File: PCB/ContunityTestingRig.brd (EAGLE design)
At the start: 82.8 x 65 mm, 29 parts

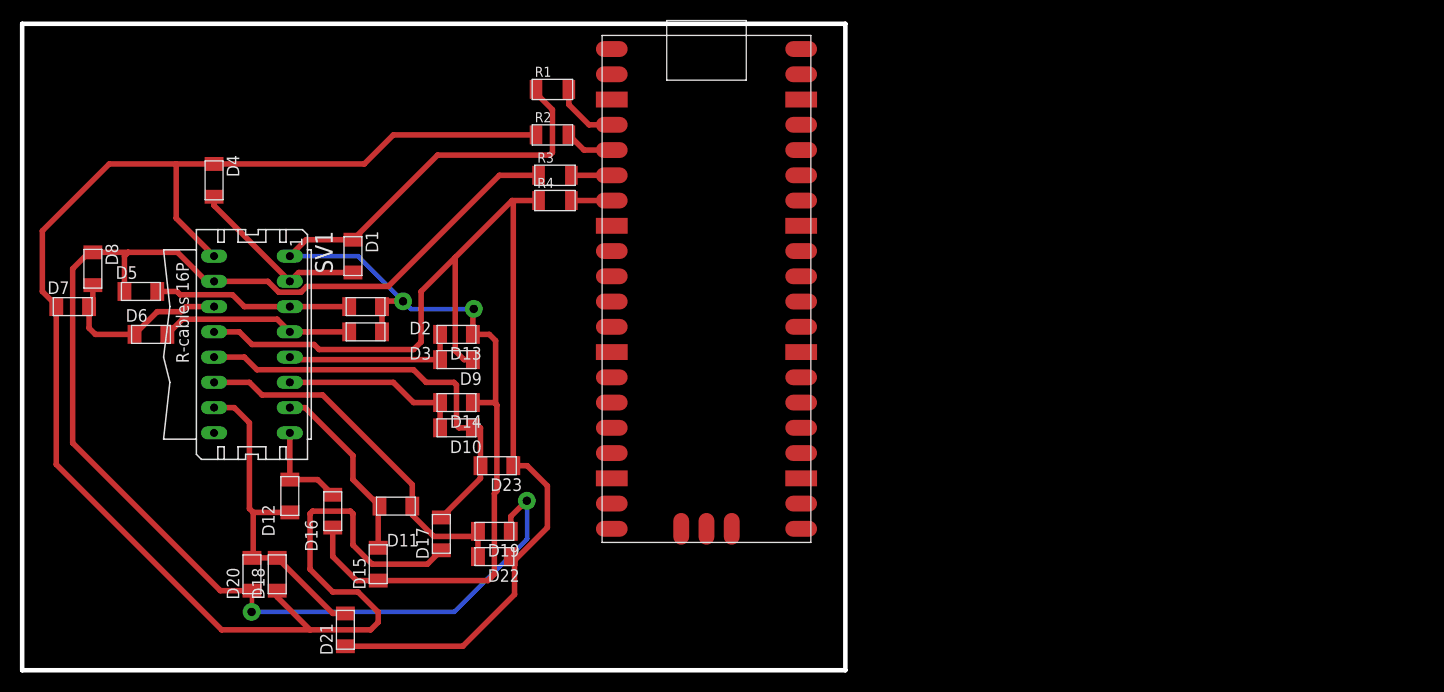
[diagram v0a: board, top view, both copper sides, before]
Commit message: Updates
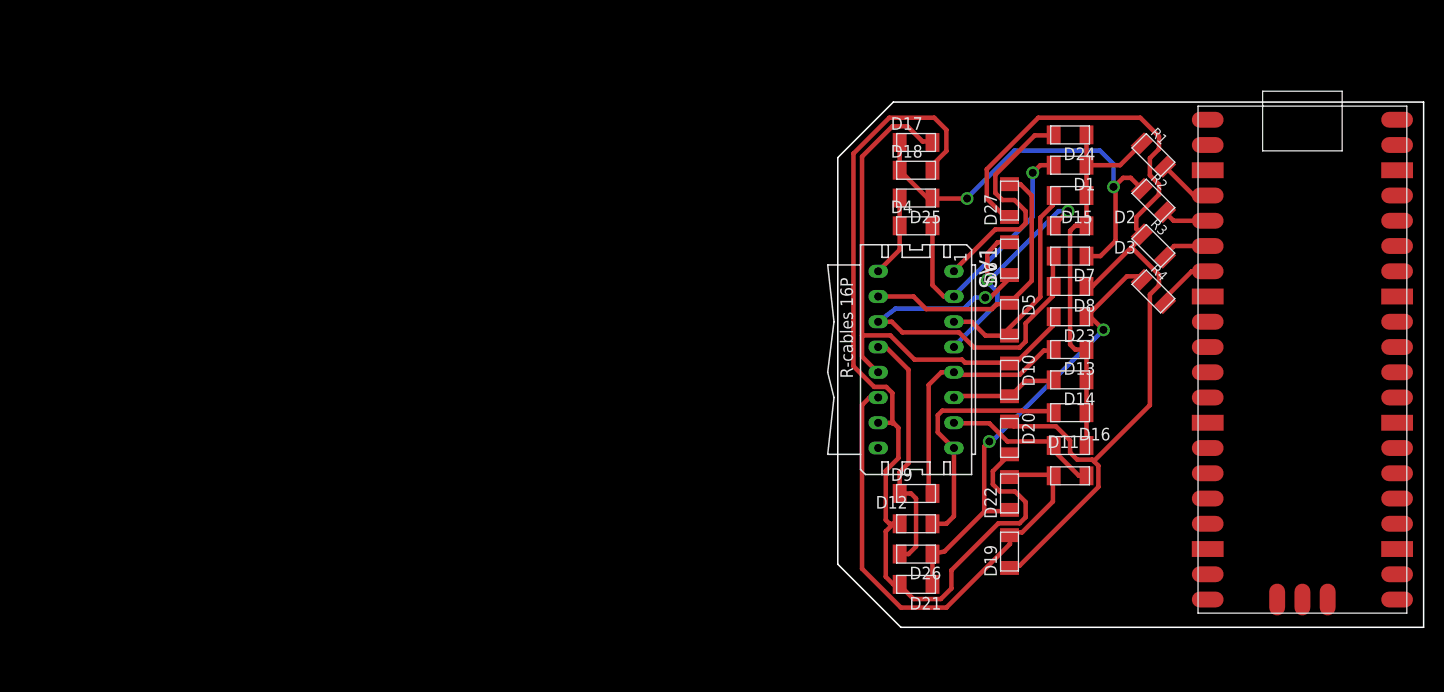
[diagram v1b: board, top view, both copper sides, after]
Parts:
- added D24, D25, D26, D27: SCHOTTKY, eagle_fab:MINI-SMA
- moved D7 100.5 mm to (110.2, 47.0), turned to 180 degrees
- moved D8 98.3 mm to (110.2, 43.9), turned to 180 degrees
- moved D5 87.4 mm to (104.1, 40.6), turned to 270 degrees
- moved D6 86.7 mm to (104.1, 46.7), turned to 90 degrees
- moved D20 77.4 mm to (104.1, 28.7), turned to 270 degrees
- moved D18 76.0 mm to (94.7, 55.6), turned to 0 degrees
- moved D16 74.8 mm to (110.2, 31.2), turned to 180 degrees
- moved D1 72.7 mm to (110.2, 56.1), turned to 180 degrees
- moved D2 71.7 mm to (110.2, 53.1)
- moved D3 71.7 mm to (110.2, 50.0)
- moved D4 70.8 mm to (94.7, 50.0), turned to 0 degrees
- moved D15 70.6 mm to (110.2, 27.9), turned to 180 degrees
- moved D11 67.9 mm to (110.2, 24.9), turned to 0 degrees
- moved SV1 66.8 mm to (94.7, 36.6)
- moved D12 63.1 mm to (94.7, 20.1), turned to 0 degrees
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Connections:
- new net N$10: D24.ANODE, SV1.1
- new net N$11: D25.ANODE, D4.KATHODE, SV1.2
- new net N$12: D26.ANODE, D9.KATHODE, SV1.8
- new net N$13: D27.ANODE, D5.KATHODE, SV1.4
- net 1: now also D24.KATHODE; no longer SV1.1
- net 4: now also D25.KATHODE; no longer D4.KATHODE, SV1.2
- net 8: now also D26.KATHODE; no longer D9.KATHODE, SV1.8
- net N$6: now also D27.KATHODE; no longer D5.KATHODE, SV1.4
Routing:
- net 4: track 166.7 -> 43.1 mm, vias 0 -> 2
- net 1: track 115.2 -> 40.4 mm
- net 8: track 117.7 -> 45.6 mm, vias 0 -> 2
- net 14: track 33.4 -> 93.6 mm
- net N$9: track 34.6 -> 0.00 mm, vias 1 -> 0
- net N$13: track 0.00 -> 28.4 mm
- net N$12: track 0.00 -> 25.5 mm
- net N$10: track 0.00 -> 23.6 mm
- net 6: track 18.5 -> 41.2 mm, vias 0 -> 1
- net 15: track 9.65 -> 25.3 mm
- net 12: track 37.5 -> 51.6 mm
- net 10: track 42.8 -> 54.3 mm
- net N$6: track 105.7 -> 97.3 mm
- net 3: track 18.4 -> 26.8 mm, vias 0 -> 1
- net N$11: track 0.00 -> 8.26 mm
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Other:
- board size 82.8 x 65 mm -> 58.9 x 52.8 mm
